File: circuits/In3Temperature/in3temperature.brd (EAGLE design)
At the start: 45.4 x 39.3 mm, 24 parts, among them IC1 ATMEGA48/88/168-AU, Q1 MOSFET-NCHANNELSMD, Q2 MOSFET-NCHANNELSMD, Q3 MOSFET-NCHANNELSMD, Q4 MOSFET-NCHANNELSMD, Q5 MOSFET-NCHANNELSMD

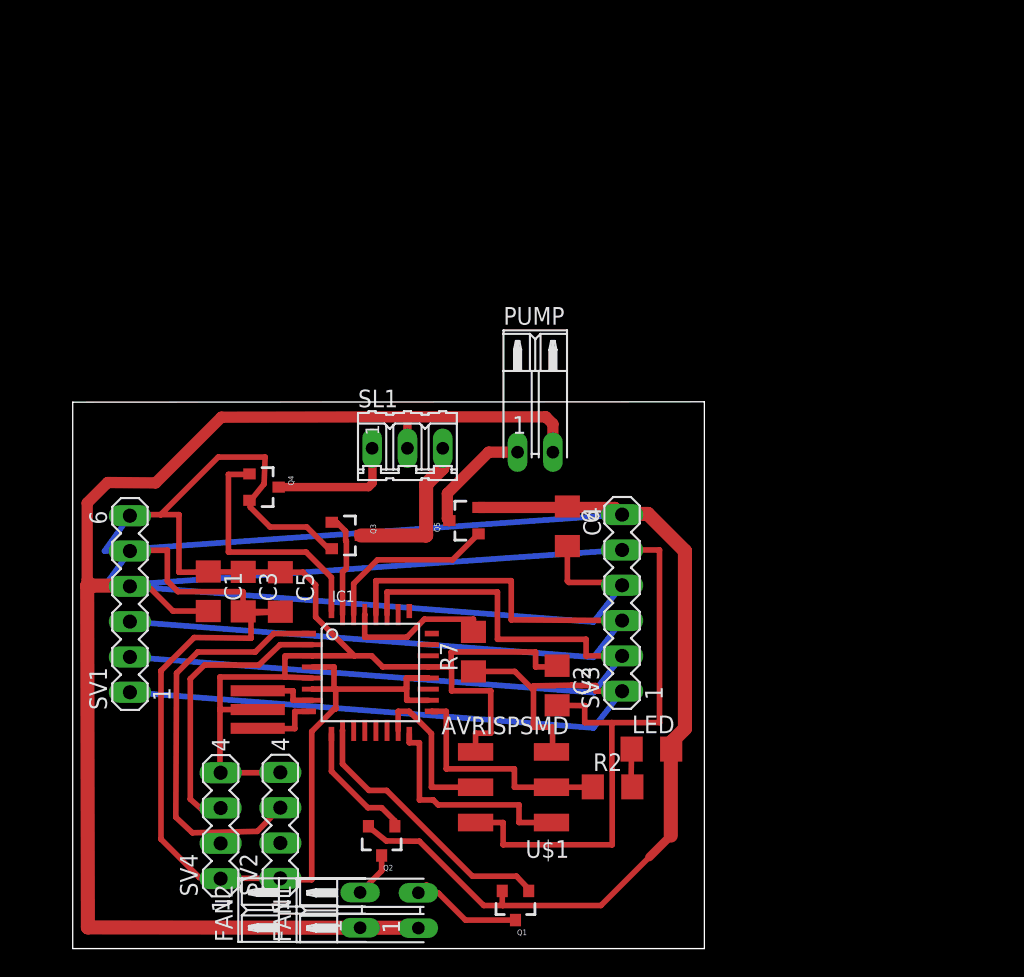
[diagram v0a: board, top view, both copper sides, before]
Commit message: Electronics v2
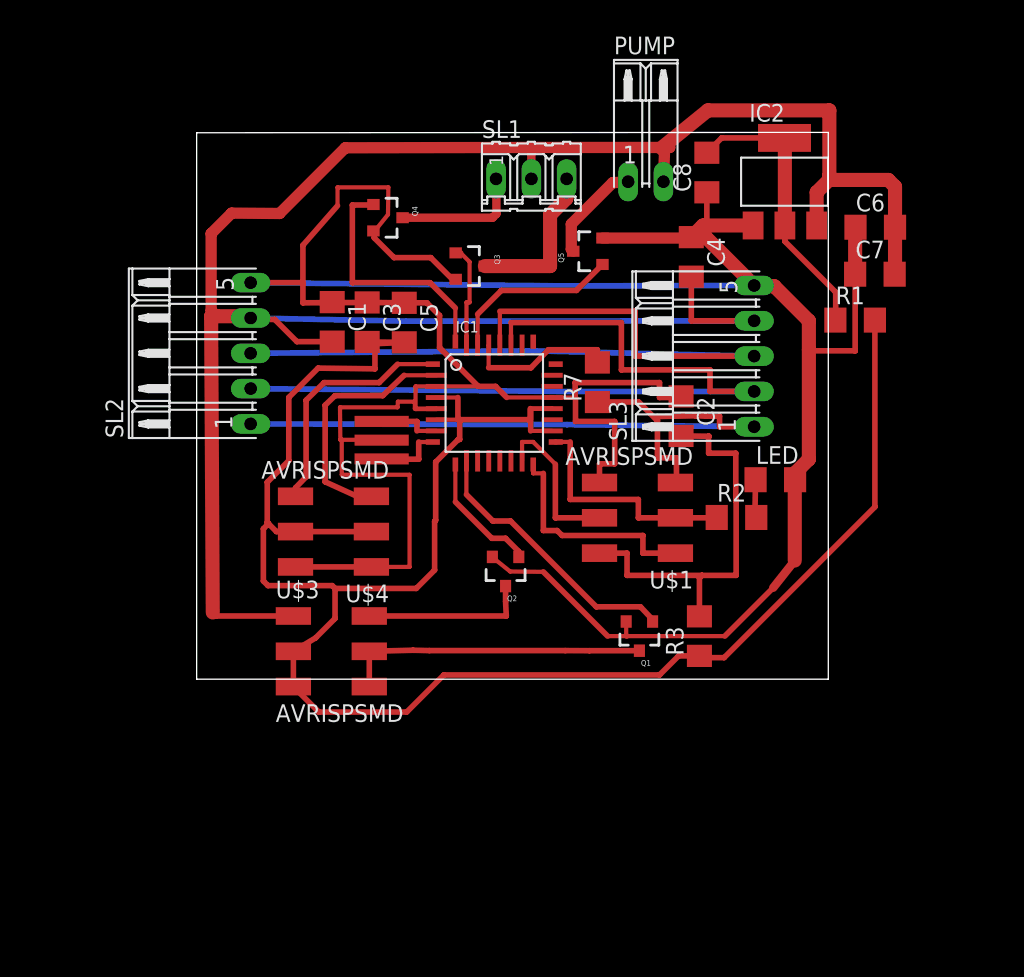
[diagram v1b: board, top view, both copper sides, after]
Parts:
- removed FAN1, FAN2: (no value), con-amp-quick:02PA
- removed SV1, SV3: (no value), con-lstb:MA06-1
- removed SV2, SV4: (no value), con-lstb:MA04-1
- added C6, C8: 10uf, ng:1206
- added C7: .1uf, ng:1206
- added IC2: REG1117, burr-brown:SOT223
- added R1, R3: 0, ng:1206
- added SL2, SL3: (no value), con-amp-quick:05PA
- added U$3, U$4: AVRISPSMD, 01_FAB_Hello:2X03SMD
- moved C2 21.3 mm to (43.8, 38.3)
- moved C3 21.3 mm to (21.2, 45.1)
- moved C5 21.3 mm to (23.9, 45.1)
- moved LED 21.3 mm to (50.6, 33.8)
- moved Q3 21.3 mm to (28.6, 49.1)
- moved Q4 21.3 mm to (22.7, 52.6)
- moved R7 21.3 mm to (37.8, 40.8)
- moved U$1 21.3 mm to (40.9, 31.0)
- moved C1 21.3 mm to (18.7, 45.1)
- moved C4 21.3 mm to (44.6, 49.8)
- moved IC1 21.3 mm to (30.4, 39.3)
- moved Q1 21.3 mm to (40.8, 22.6)
- moved Q2 21.3 mm to (31.2, 27.2)
- moved Q5 21.3 mm to (37.2, 50.2)
- moved R2 21.3 mm to (47.8, 31.0)
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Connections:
- net 12V: now also C6.2, C7.2, IC2.3, SL2.4, SL3.4, U$3.1; no longer FAN1.1, FAN2.1, SV1.4, SV3.4
- net 5V: now also C8.2, IC2.2, R1.1, R1.2, R3.1, R3.2, U$3.3, U$3.5, U$4.3, U$4.4; no longer SV1.5, SV2.1, SV3.5, SV4.1
- net FAN1O: now also U$3.4, U$3.6; no longer FAN1.2
- net FAN2O: now also U$3.2; no longer FAN2.2
- net GND: now also C6.1, C7.1, C8.1, IC2.1, SL2.5, SL3.5, U$4.1, U$4.2; no longer SV1.6, SV2.4, SV3.6, SV4.4
- net PD3: now also U$4.6; no longer SV2.3
- net PD4: now also U$4.5; no longer SV4.3
- net RST: now also SL2.1, SL3.1; no longer SV1.1, SV3.1
- net SCL: now also SL2.3, SL3.3; no longer SV1.3, SV3.3
- net SDA: now also SL2.2, SL3.2; no longer SV1.2, SV3.2
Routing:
- net 5V: track 166.3 -> 197.0 mm
- net GND: track 205.4 -> 234.0 mm
- net FAN1O: track 8.62 -> 22.0 mm
- net 12V: track 148.1 -> 160.6 mm
- net PD3: track 29.8 -> 17.4 mm
- net FAN2O: track 3.30 -> 12.0 mm
- net PD4: track 20.9 -> 17.9 mm
- net N$3: track 8.30 -> 7.34 mm

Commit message: New Electronics
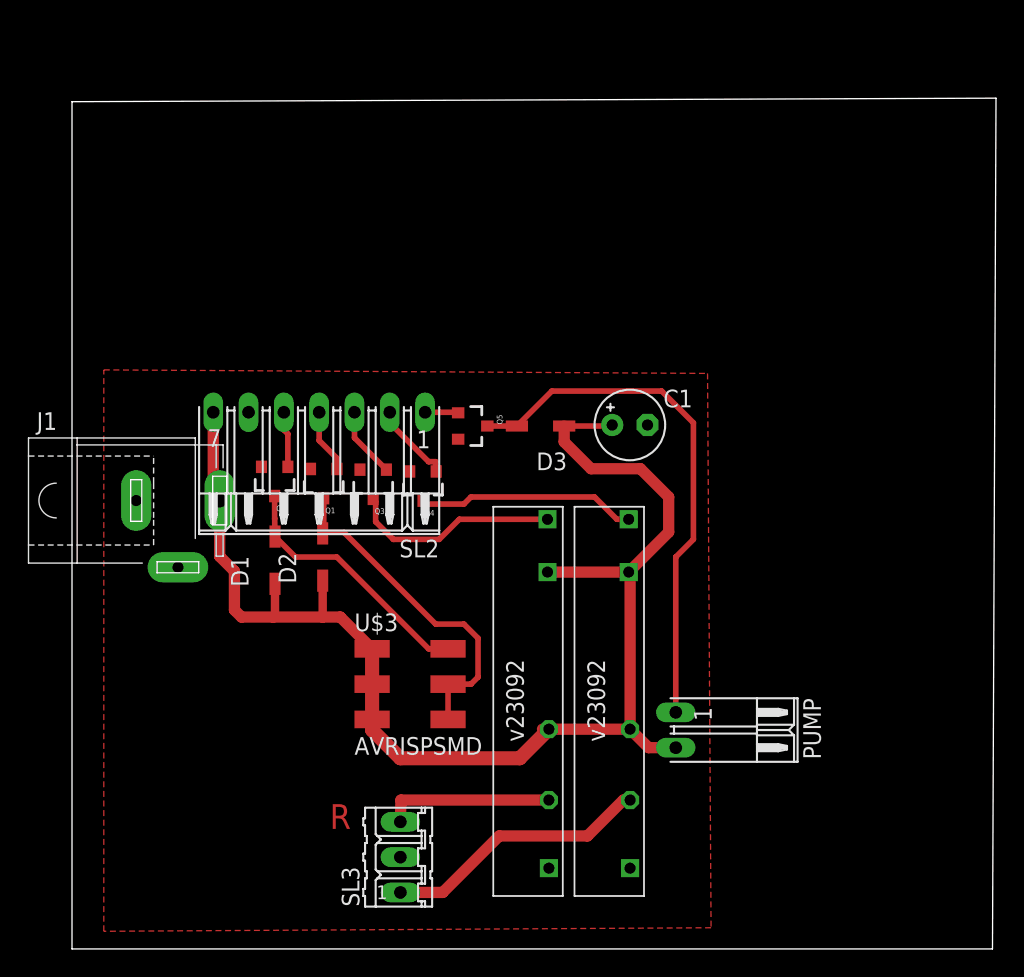
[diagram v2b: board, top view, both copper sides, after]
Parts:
- removed C2: 1uf, ng:1206
- removed C3, C7: .1uf, ng:1206
- removed C4, C5, C6, C8: 10uf, ng:1206
- removed IC1: ATMEGA48/88/168-AU, atmega8:TQFP32-08
- removed IC2: REG1117, burr-brown:SOT223
- removed LED: (no value), ng:1206
- removed R1, R3, R7: 0, ng:1206
- removed R2: 499, ng:1206
- removed SL1: (no value), con-amp-quick:03P
- removed U$4: AVRISPSMD, 01_FAB_Hello:2X03SMD
- added D1, D2, D3: (no value), fab:SOD123
- added J1: (no value), con-jack:SPC4078
- C1: value 1uf -> (none); device ng:1206 -> resistor:E2,5-5
- SL2: device con-amp-quick:05PA -> con-amp-quick:07PA
- SL3: device con-amp-quick:05PA -> con-amp-quick:03P
- U$1: value AVRISPSMD -> RELAY-V23092THROUGH_HOLE; device 01_FAB_Hello:2X03SMD -> 0001_alejandro:RELAY-V23092
- U$2: value RESONATOREFOB -> RELAY-V23092THROUGH_HOLE; device fab:EFOBM -> 0001_alejandro:RELAY-V23092
- moved SL3 44.1 mm to (23.6, 6.60)
- moved PUMP 39.5 mm to (43.4, 15.7), turned to 270 degrees
- moved U$2 37.8 mm to (41.1, 3.81)
- moved U$1 27.8 mm to (35.3, 3.81), turned to 90 degrees
- moved Q1 25.2 mm to (18.1, 33.5)
- moved C1 22.7 mm to (40.1, 37.7), turned to 0 degrees
- moved Q4 19.4 mm to (25.2, 33.4), turned to 180 degrees
- moved Q2 17.8 mm to (14.6, 33.7)
- moved Q3 17.1 mm to (21.7, 33.5), turned to 180 degrees
- moved Q5 15.1 mm to (28.8, 37.6), turned to 270 degrees
- moved SL2 6.50 mm to (17.8, 38.6), turned to 180 degrees
- moved U$3 6.14 mm to (24.1, 19.1)
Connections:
- removed net 5V: C2.2, C3.2, C5.2, C8.2, IC1.18, IC1.20, IC1.4, IC1.6, IC2.2, R1.1, R1.2, R3.1, R3.2, U$1.2, U$3.3, U$3.5, U$4.3, U$4.4
- removed net FAN1: IC1.10, Q1.1
- removed net FAN2: IC1.9, Q2.1
- removed net MISO: IC1.16, U$1.1
- removed net MOSI: IC1.15, U$1.4
- removed net N$1: IC1.8, U$2.1
- removed net N$23: LED.1, R2.2
- removed net N$9: IC1.7, U$2.3
- removed net PD0: IC1.30, Q5.1
- removed net PD3: IC1.1, U$4.6
- removed net PD4: IC1.2, U$4.5
- removed net RST: IC1.29, R7.1, R7.2, SL2.1, SL3.1, U$1.5
- removed net SCK: IC1.17, R2.1, U$1.3
- removed net SCL: IC1.28, SL2.3, SL3.3
- removed net SDA: IC1.27, SL2.2, SL3.2
- new net BLACK: SL3.1, U$2.3
- new net FAN12: Q2.1, SL2.5
- new net FAN5: Q1.1, SL2.4
- new net PUMP: Q5.1, SL2.1
- new net RED: SL3.3, U$1.3
- net 12V: now also C1.+, D1.CATHODE, D2.CATHODE, D3.CATHODE, J1.3, SL2.7, U$1.2, U$1.4, U$2.2, U$2.4, U$3.3, U$3.5; no longer C1.2, C4.2, C6.2, C7.2, IC2.3, SL1.2, SL2.4, SL3.4
- net FAN1O: now also D2.ANODE
- net FAN2O: now also D1.ANODE
- net GND: now also C1.-, J1.1, J1.2, SL2.6, U$1.1, U$2.1; no longer C1.1, C2.1, C3.1, C4.1, C5.1, C6.1, C7.1, C8.1, IC1.21, IC1.3, IC1.5, IC2.1, LED.2, SL2.5, SL3.5, U$1.6, U$2.2, U$4.1, U$4.2
- net N$3: now also D3.ANODE
- net RELAY1: now also SL2.3; no longer IC1.31
- net RELAY1O: now also U$1.5; no longer SL1.3
- net RELAY2: now also SL2.2; no longer IC1.32
- net RELAY2O: now also U$2.5; no longer SL1.1
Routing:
- net GND: track 234.0 -> 0.00 mm
- net 5V: track 197.0 -> 0.00 mm
- net RST: track 66.0 -> 0.00 mm
- net 12V: track 160.6 -> 99.7 mm
- net SDA: track 60.3 -> 0.00 mm
- net SCL: track 60.2 -> 0.00 mm
- net N$3: track 7.34 -> 38.2 mm
- net FAN1: track 19.7 -> 0.00 mm
- net BLACK: track 0.00 -> 19.3 mm
- net PD4: track 17.9 -> 0.00 mm
- net PD3: track 17.4 -> 0.00 mm
- net SCK: track 17.1 -> 0.00 mm
- net MISO: track 16.4 -> 0.00 mm
- net PD0: track 12.7 -> 0.00 mm
- net RED: track 0.00 -> 12.2 mm
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- added copper zone on layer 1, net GND
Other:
- board size 45.4 x 39.3 mm -> 66.5 x 61.2 mm
- board text added: "R"
